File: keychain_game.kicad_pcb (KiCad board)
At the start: 2 copper layers, 26.8 x 26.8 mm, 28 parts, among them J1 Conn_02x03_Counter_Clockwise, J2 Conn_01x02, SW1 SW_MEC_5G, U1 MIC5205-2.5, U2 SN74HC595DR, U4 ATTINY13A-MMF

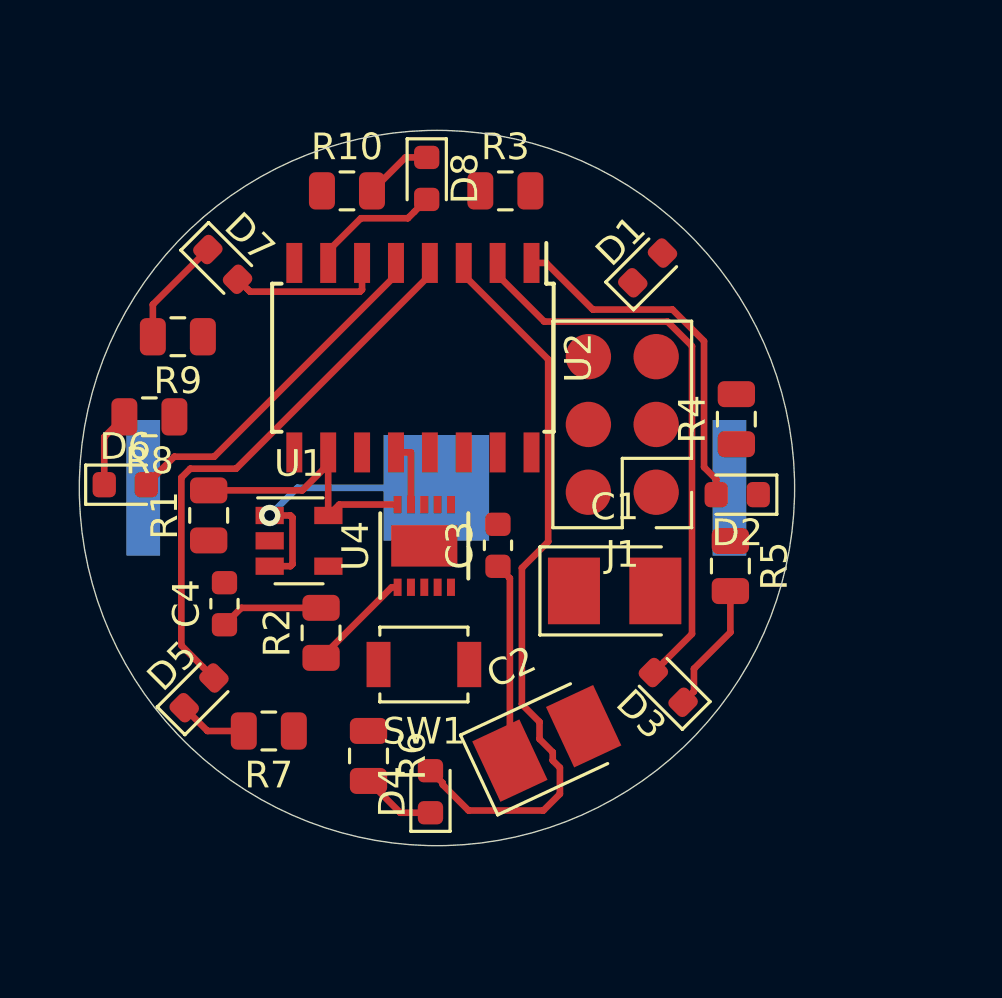
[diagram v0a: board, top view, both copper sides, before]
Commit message: finished board
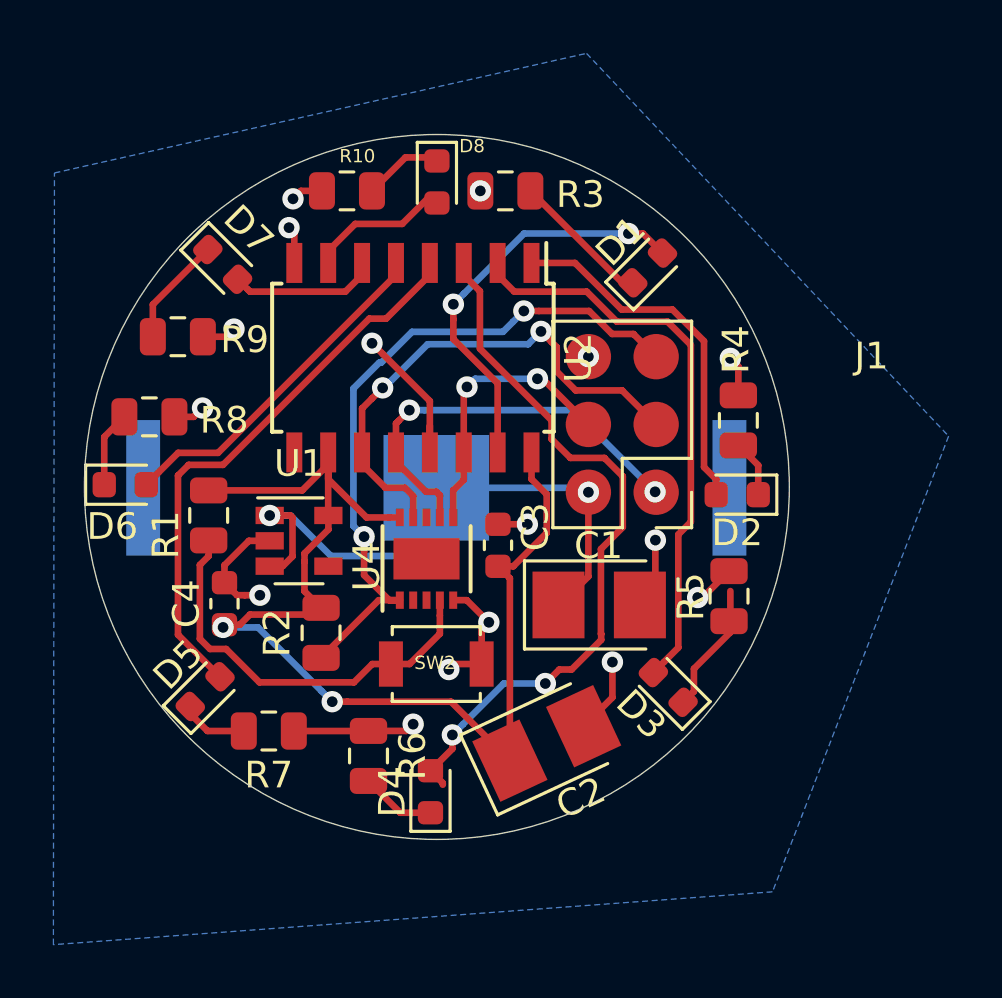
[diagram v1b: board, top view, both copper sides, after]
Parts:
- removed SW1: SW_MEC_5G, Button_Switch_SMD:SW_SPST_B3U-1000P
- added SW2: SW_DPST_x2, Button_Switch_SMD:SW_SPST_B3U-1000P, F.Cu at (149.1, 99.0)
- moved R5 1.13 mm to (160.0, 96.5)
- moved C1 0.78 mm to (155.2, 96.8)
- moved U4 0.49 mm to (148.7, 95.1)
- moved D8 0.40 mm to (149.1, 81.0)
- moved D5 0.23 mm to (140.4, 100.1)
- moved R4 0.09 mm to (160.4, 89.9), turned to 270 degrees
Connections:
- J1 pad 3: RCLK -> SCK
- U2 pad 11: MISO -> SCK
- U2 pad 12: RCLK -> MISO
- U4 pad 9: RCLK -> SCK
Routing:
- net GND: track 0.00 -> 33.5 mm, vias 0 -> 16
- net +2V5: track 21.8 -> 46.0 mm, vias 0 -> 2
- net RESET: track 3.96 -> 26.0 mm, vias 0 -> 2
- net SCK: track 0.00 -> 19.2 mm, vias 0 -> 2
- net Net-(R1-Pad1): track 0.00 -> 15.5 mm
- net Net-(D1-Pad2): track 0.00 -> 15.5 mm, vias 0 -> 2
- net MISO: track 0.00 -> 15.4 mm, vias 0 -> 2
- net VCC: track 10.2 -> 22.3 mm, vias 1 -> 2
- net MOSI: track 0.00 -> 10.5 mm, vias 0 -> 2
- net Net-(D1-Pad1): track 0.00 -> 5.26 mm
- net RCLK: track 2.51 -> 0.00 mm
- net Net-(D2-Pad1): track 0.00 -> 2.16 mm
- net Net-(D4-Pad2): track 28.0 -> 27.1 mm, vias 0 -> 2
- added copper zone on B.Cu, net GND
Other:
- board size 26.8 x 26.8 mm -> 26.4 x 26.4 mm
